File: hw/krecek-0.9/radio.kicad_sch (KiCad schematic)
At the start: 19 parts, among them J4 U.FL, U11 CC1101RGPR

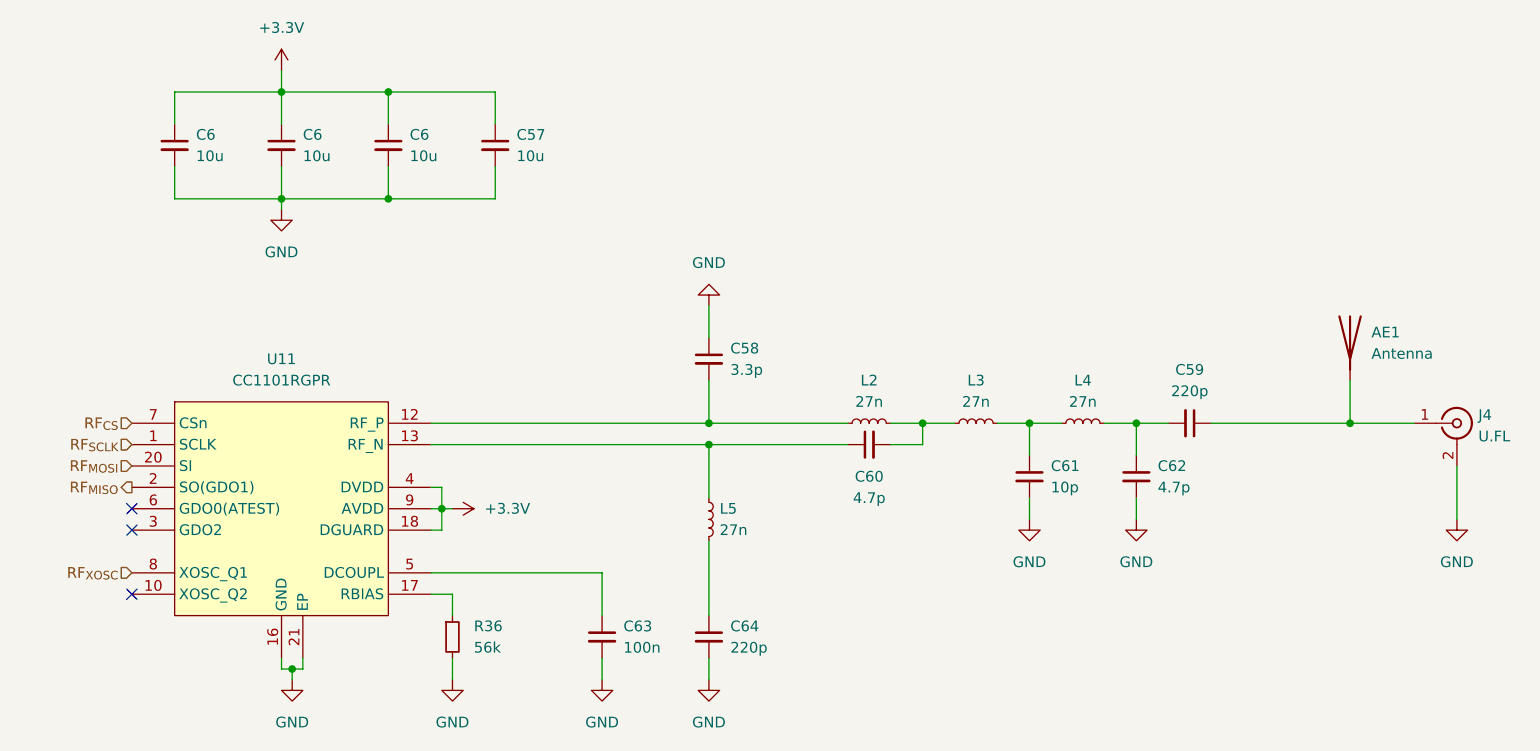
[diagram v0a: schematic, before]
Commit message: Work on board layout
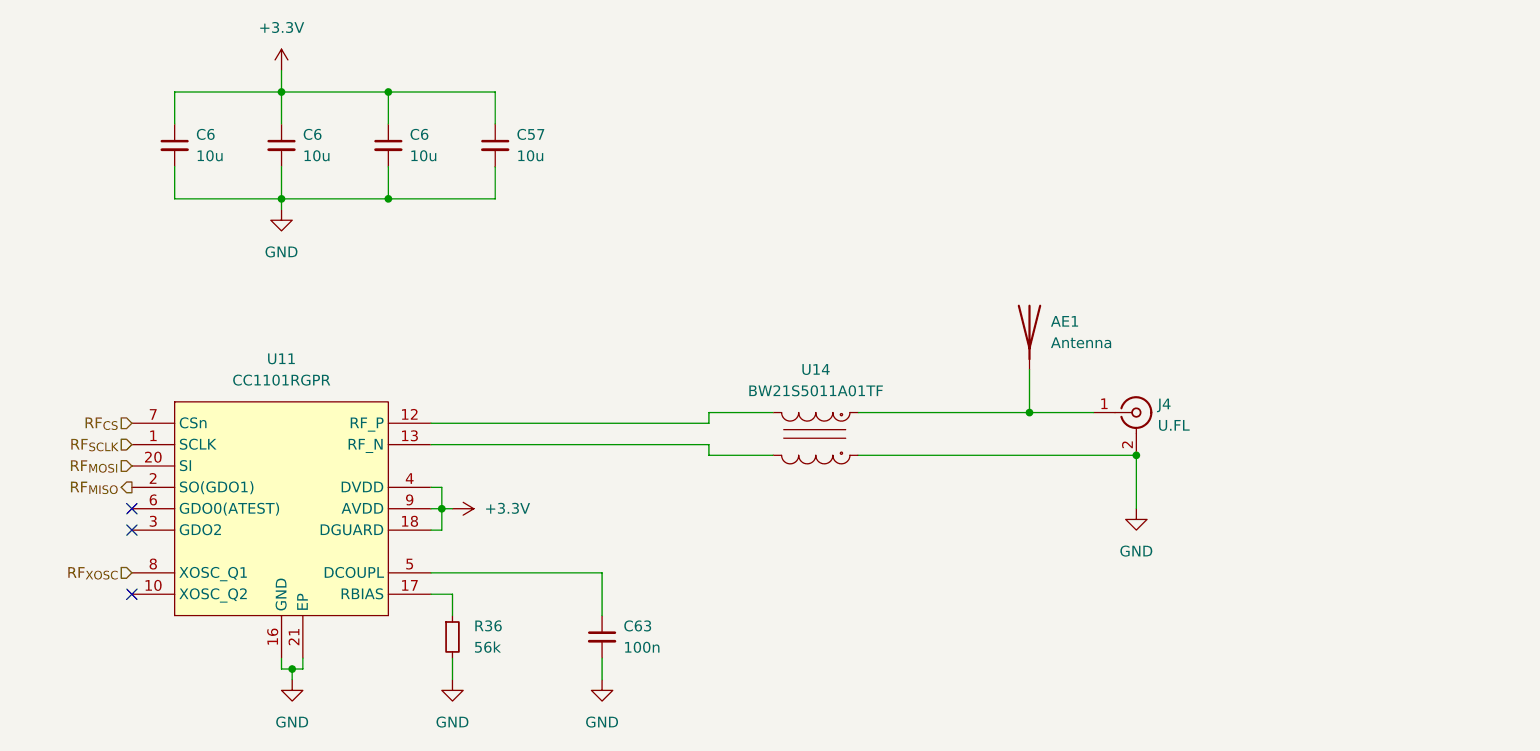
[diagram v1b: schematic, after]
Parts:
- removed C58: 3.3p, Capacitor_SMD:C_0402_1005Metric, symbol Device:C_Small
- removed C59, C64: 220p, Capacitor_SMD:C_0402_1005Metric, symbol Device:C_Small
- removed C60, C62: 4.7p, Capacitor_SMD:C_0402_1005Metric, symbol Device:C_Small
- removed C61: 10p, Capacitor_SMD:C_0402_1005Metric, symbol Device:C_Small
- removed L2, L3, L4, L5: 27n, Inductor_SMD:L_0402_1005Metric, symbol Device:L_Small
- added U14: BW21S5011A01TF, LCSC:FILTER-SMD_4P-L2.0-W1.2-BL-1, symbol LCSC:BW21S5011A01TF
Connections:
- net GND: now also U14.1
- net at U11.12 (RF_P): now also U14.3
- net at AE1.1 (A), J4.1 (In): now also U14.4
- net at U11.13 (RF_N): now also U14.2
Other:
- moved on the sheet: AE1, J4
